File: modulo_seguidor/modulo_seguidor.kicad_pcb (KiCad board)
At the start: 2 copper layers, 140 x 90 mm, 26 parts, among them J1 Battery, J6 puerto sensores, M1 Motor_IZQ, M2 Motor_DER, SW1 SW_Push, SW2 SW_Nidec_CAS-120A1, U1 LM7806_TO220, U2 L298N

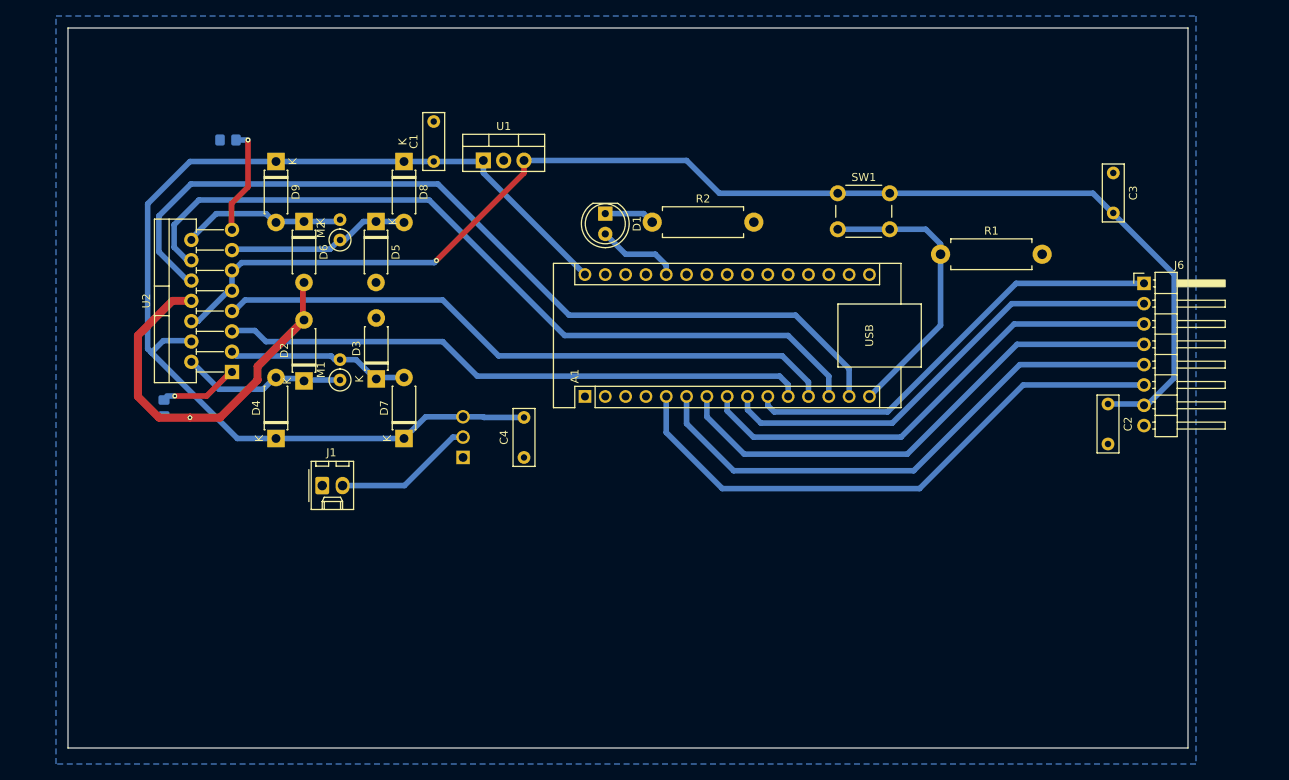
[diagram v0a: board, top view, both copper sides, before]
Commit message: refactor!(modulo-seguidor): Modifico forma de la placa
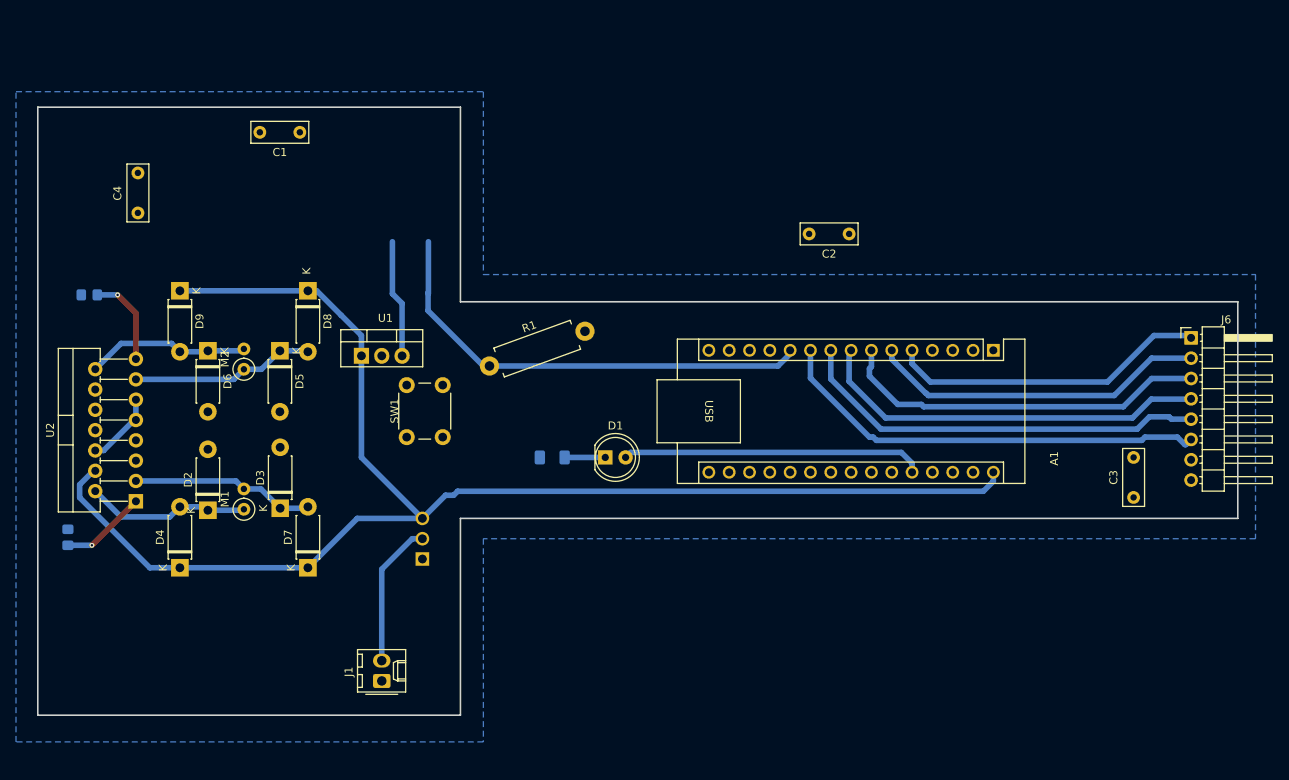
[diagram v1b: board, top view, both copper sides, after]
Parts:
- R2: footprint Resistor_THT:R_Axial_DIN0411_L9.9mm_D3.6mm_P12.70mm_Horizontal -> Resistor_SMD:R_1206_3216Metric_Pad1.30x1.75mm_HandSolder; moved to B.Cu
- moved SW1 61.9 mm to (112.3, 104.1), turned to 90 degrees
- moved R1 58.1 mm to (122.7, 95.2), turned to 20 degrees
- moved C4 57.1 mm to (78.7, 76.1)
- moved A1 51.4 mm to (185.7, 93.3), turned to -90 degrees
- moved C3 40.6 mm to (203.2, 111.7), turned to 90 degrees
- moved C2 38.7 mm to (167.6, 78.7), turned to 180 degrees
- moved R2 32.0 mm to (130.5, 106.7), turned to 180 degrees
- moved D1 30.5 mm to (137.2, 106.7), turned to 0 degrees
- moved U1 28.8 mm to (106.7, 94.0)
- moved R4 26.0 mm to (72.7, 86.4)
- moved J1 25.5 mm to (109.2, 134.6), turned to 90 degrees
- moved D2 20.1 mm to (87.5, 113.3)
- moved D3 20.1 mm to (96.5, 113.0)
- moved D4 20.1 mm to (84.0, 120.5)
- moved D5 20.1 mm to (96.5, 93.4)
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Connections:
- A1 pad 11: /Entrada PWM Motor A -> /Boton_encendido
- A1 pad 12: /Entrada DIG Motor A -> /Entrada PWM Motor A
- A1 pad 13: /Entrada DIG Motor B -> /Entrada DIG Motor A
- A1 pad 14: /Entrada PWM Motor B -> /Entrada DIG Motor B
- A1 pad 15: /Boton_encendido -> /Entrada PWM Motor B
- J6 pad 1: /Sensor6 -> /Sensor1
- J6 pad 2: /Sensor5 -> /Sensor2
- J6 pad 3: /Sensor4 -> /Sensor3
- J6 pad 4: /Sensor3 -> /Sensor4
- J6 pad 5: /Sensor2 -> /Sensor5
- J6 pad 6: /Sensor1 -> /Sensor6
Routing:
- net Salida Regulador: track 161.1 -> 24.0 mm, vias 1 -> 0
- net /Entrada PWM Motor B: track 110.9 -> 0.00 mm
- net /Entrada DIG Motor B: track 100.3 -> 0.00 mm
- net /Entrada DIG Motor A: track 78.7 -> 0.00 mm
- net /Entrada PWM Motor A: track 73.9 -> 0.00 mm
- net GND: track 49.2 -> 0.05 mm, vias 1 -> 0
- net VCC: track 140.5 -> 178.8 mm
- net /Sensor1: track 72.5 -> 40.0 mm
- net Net-(A1-A7): track 10.4 -> 37.8 mm
- net /Sensor2: track 68.5 -> 42.3 mm
- net /Boton_encendido: track 36.3 -> 58.0 mm
- net /Sensor3: track 64.8 -> 46.6 mm
- net /Sensor4: track 61.1 -> 49.6 mm
- net /Sensor5: track 58.1 -> 52.0 mm
- net Net-(U2-SENSE_B): track 13.5 -> 11.5 mm
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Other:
- board size 140 x 90 mm -> 150 x 76 mm
